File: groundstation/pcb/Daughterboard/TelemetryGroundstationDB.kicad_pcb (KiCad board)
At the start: 2 copper layers, 40 x 70 mm, 32 parts, among them J1 RFPC-SMA27-F, J2 ICD15S13E4GV00LF, M1 M4 Mounting Hole, M2 M4 Mounting Hole, M3 M4 Mounting Hole, M4 M4 Mounting Hole, U1 RC1780HP-RC232

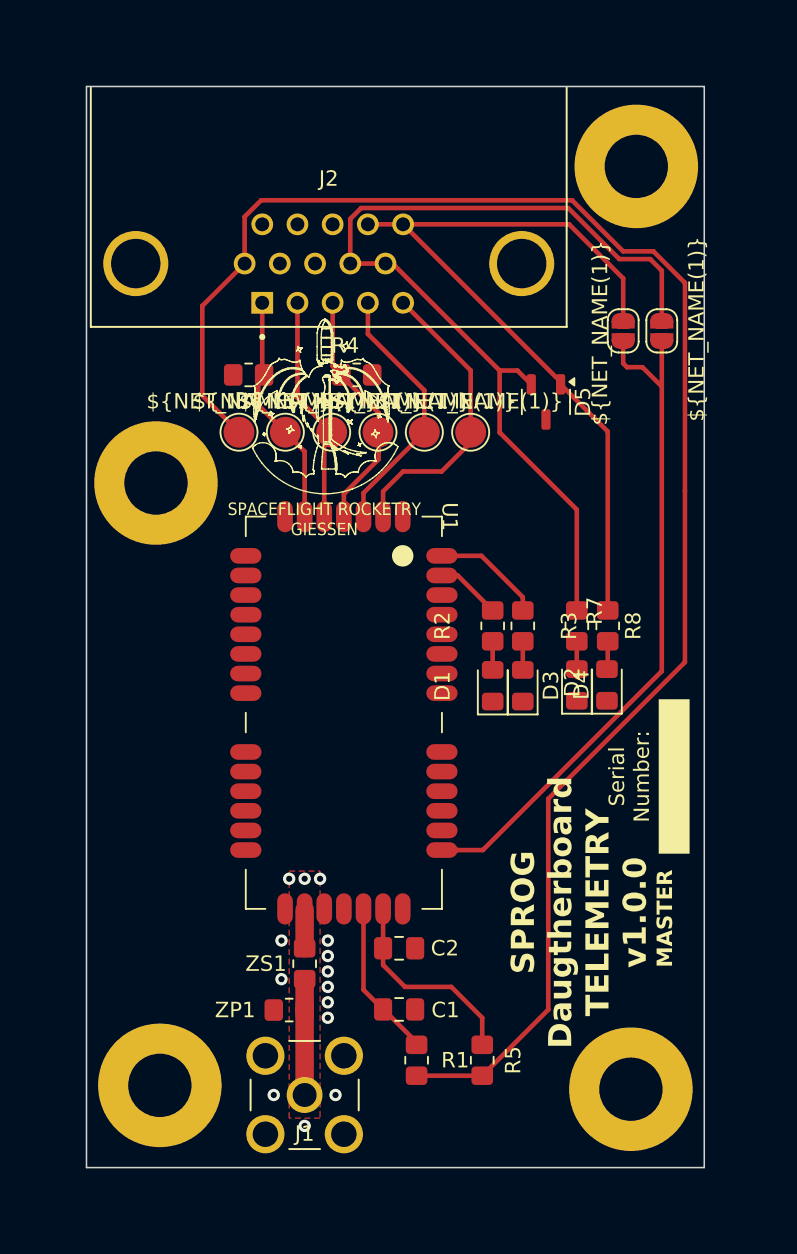
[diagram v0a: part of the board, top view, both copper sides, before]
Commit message: finalized design of daughterbaord
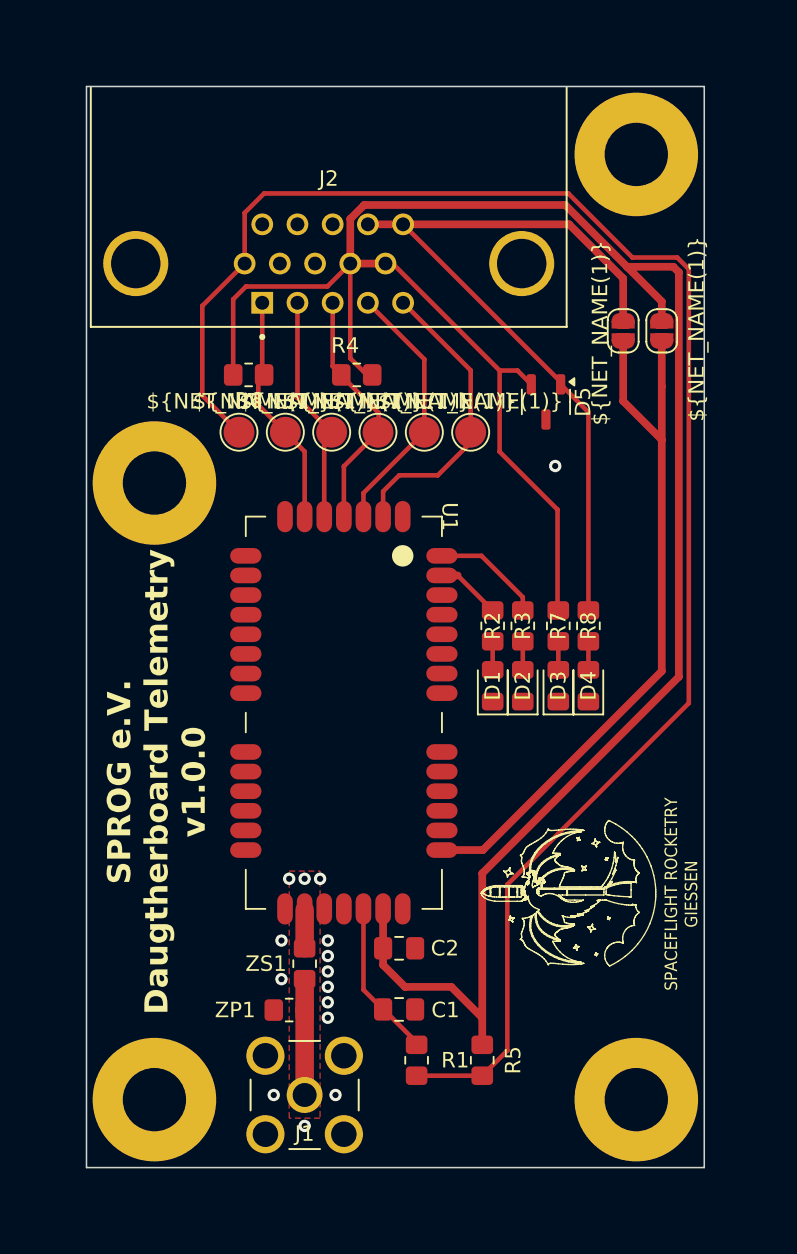
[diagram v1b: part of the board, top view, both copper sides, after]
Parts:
- moved R8 1.25 mm to (12.5, 5.00)
- moved D3 1.20 mm to (10.6, 8.88)
- moved D4 1.20 mm to (12.5, 8.88)
- moved R7 1.20 mm to (10.6, 5.00)
- moved M4 0.99 mm to (-15.6, 35.7)
- moved M2 0.77 mm to (15.6, -25.5)
- moved M1 0.76 mm to (15.6, 35.7)
- moved M3 0.10 mm to (-15.6, -4.25)
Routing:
- net +3V3: track 74.4 -> 153.1 mm
- net Net-(JP1-B): track 46.2 -> 49.0 mm
- net RST: track 108.3 -> 109.6 mm
- net +5V: track 51.2 -> 50.7 mm
- net GND: vias 14 -> 15
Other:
- board text added: "SPROG e.V. Daugtherboard Telemetry v1.0.0"
- board text removed: "MASTER"
- board text removed: "SPROG Daughterboard TELEMETRY v1.0.0"
- board text removed: "SPROG Daugtherboard TELEMETRY v1.0.0"
